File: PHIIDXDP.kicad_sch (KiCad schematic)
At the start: 45 parts, among them J1 USB_C_Receptacle_USB2.0_16P, J10 2P BT 2, J11 2P BT 3, J12 2P BT 4, J13 2P BT 5, J14 2P BT 6, J15 2P BT 7, J16 1P START, J17 EFFECT, J18 VEFX, J19 2P START, J2 1P BT 1, J20 P1 TT analog, J21 P2 TT analog, J22 LED P1 TT, J23 LED P2 TT, J24 LED P1 Console, J25 LED P2 Console, J26 LED CENTER, J28 P1 TT Encoder, J29 P2 TT Encoder, J3 1P BT 3, J4 1P BT 5, J5 1P BT 7, J6 1P BT 2, J7 1P BT 4, J8 1P BT 6, J9 2P BT 1, SW1 SW_Push, U1 AT90USB647-A, Y1 16MHz

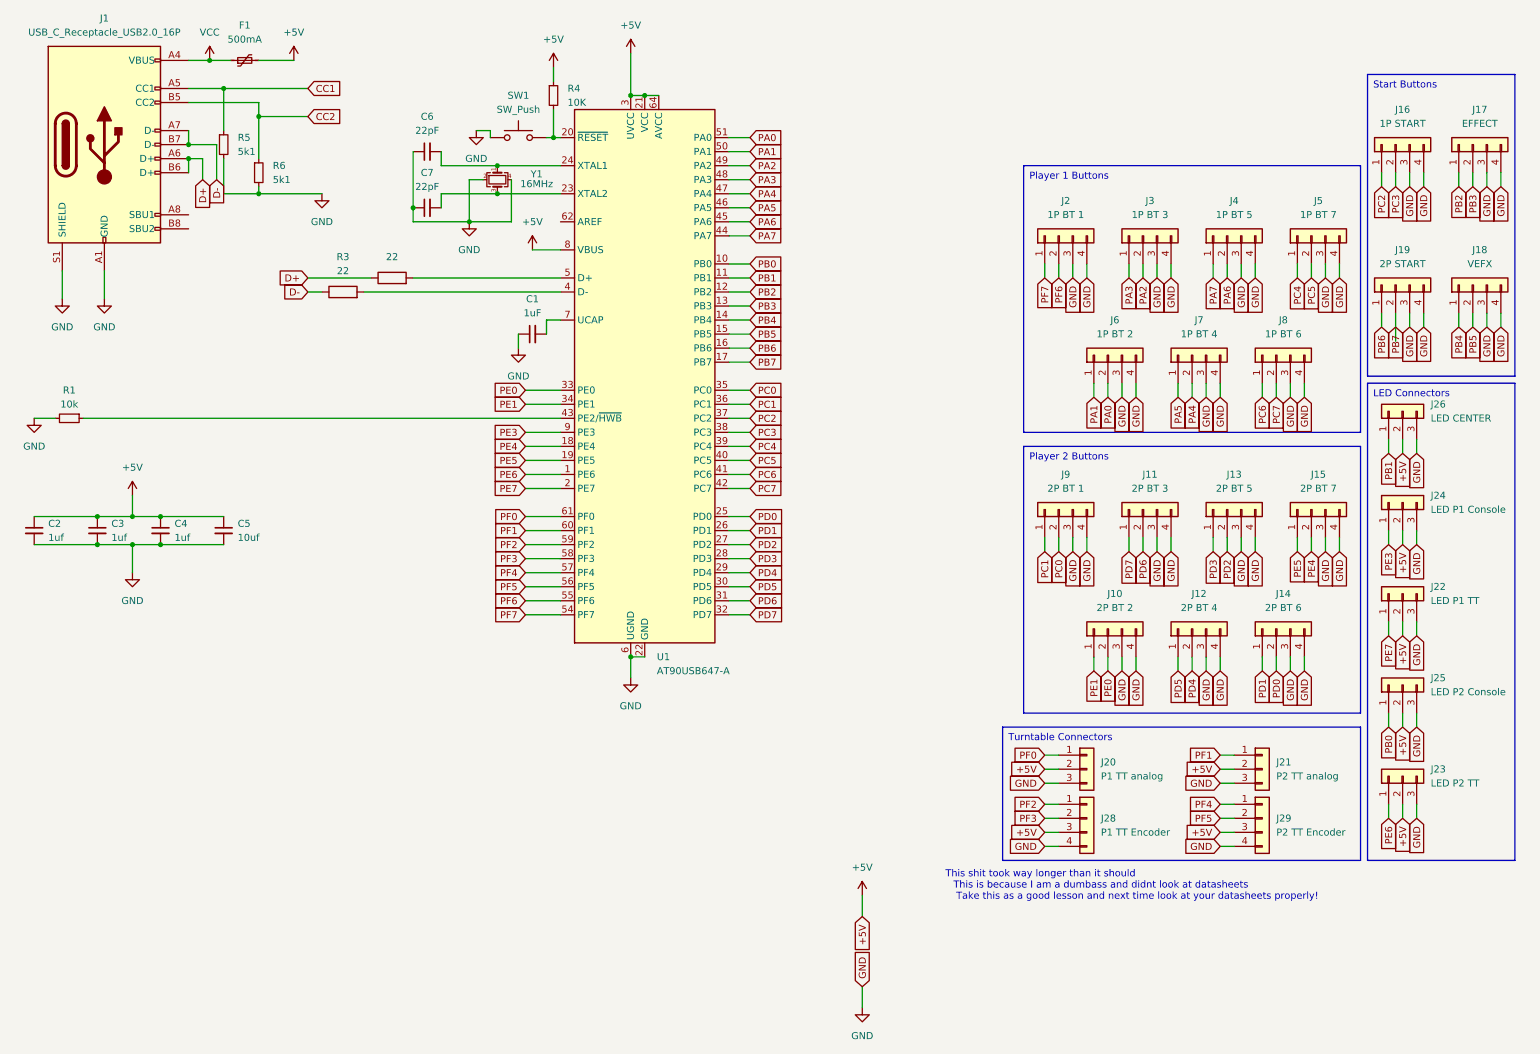
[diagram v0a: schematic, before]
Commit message: Wha?
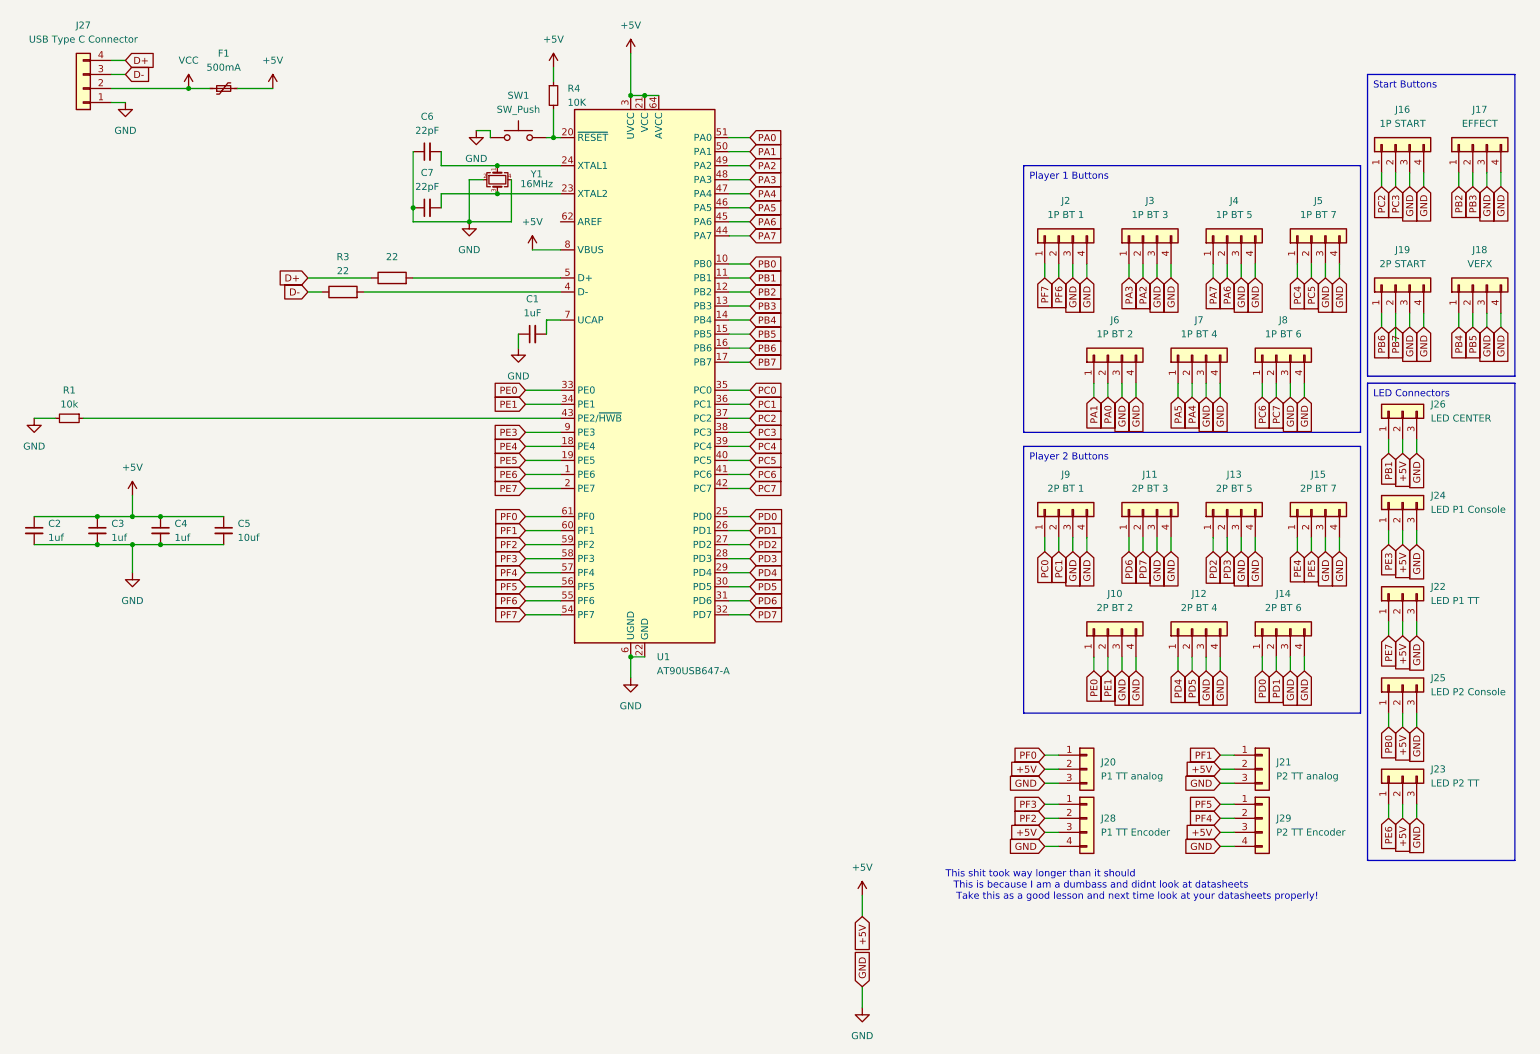
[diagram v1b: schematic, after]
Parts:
- removed J1: USB_C_Receptacle_USB2.0_16P, Connector_USB:USB_C_Receptacle_HRO_TYPE-C-31-M-12, symbol Connector:USB_C_Receptacle_USB2.0_16P
- removed R5, R6: 5k1, Resistor_SMD:R_0805_2012Metric, symbol Device:R_Small
- added J27: USB Type C Connector, Connector_JST:JST_XH_B4B-XH-AM_1x04_P2.50mm_Vertical, symbol Connector_Generic:Conn_01x04
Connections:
- net D+: now also J27.4 (Pin_4)
- net D-: now also J27.3 (Pin_3)
- net GND: now also J27.1 (Pin_1)
- net PC0: now also J9.1 (Pin_1); no longer J9.2 (Pin_2)
- net PC1: now also J9.2 (Pin_2); no longer J9.1 (Pin_1)
- net PD0: now also J14.1 (Pin_1); no longer J14.2 (Pin_2)
- net PD1: now also J14.2 (Pin_2); no longer J14.1 (Pin_1)
- net PD2: now also J13.1 (Pin_1); no longer J13.2 (Pin_2)
- net PD3: now also J13.2 (Pin_2); no longer J13.1 (Pin_1)
- net PD4: now also J12.1 (Pin_1); no longer J12.2 (Pin_2)
- net PD5: now also J12.2 (Pin_2); no longer J12.1 (Pin_1)
- net PD6: now also J11.1 (Pin_1); no longer J11.2 (Pin_2)
- net PD7: now also J11.2 (Pin_2); no longer J11.1 (Pin_1)
- net PE0: now also J10.1 (Pin_1); no longer J10.2 (Pin_2)
- net PE1: now also J10.2 (Pin_2); no longer J10.1 (Pin_1)
- net PE4: now also J15.1 (Pin_1); no longer J15.2 (Pin_2)
- net PE5: now also J15.2 (Pin_2); no longer J15.1 (Pin_1)
- net PF2: now also J28.2 (Pin_2); no longer J28.1 (Pin_1)
- net PF3: now also J28.1 (Pin_1); no longer J28.2 (Pin_2)
- net PF4: now also J29.2 (Pin_2); no longer J29.1 (Pin_1)
- net PF5: now also J29.1 (Pin_1); no longer J29.2 (Pin_2)
- net VCC: now also J27.2 (Pin_2)
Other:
- moved on the sheet: F1
